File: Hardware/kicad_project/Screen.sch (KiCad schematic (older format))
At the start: 9 parts

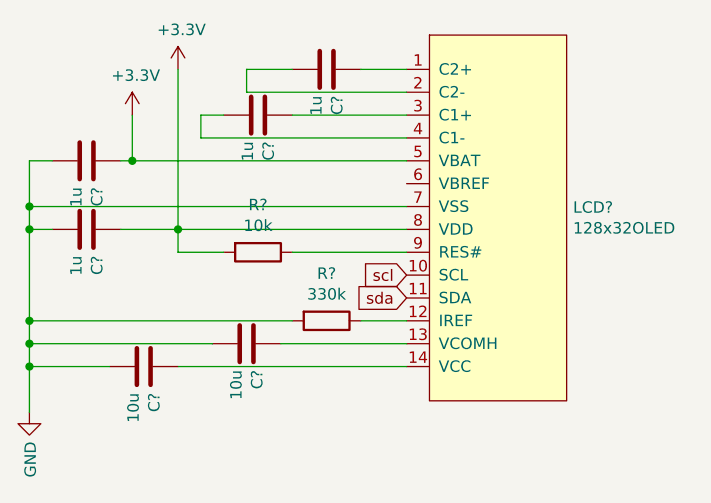
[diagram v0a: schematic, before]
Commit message: update project with corrected schematic / pcb
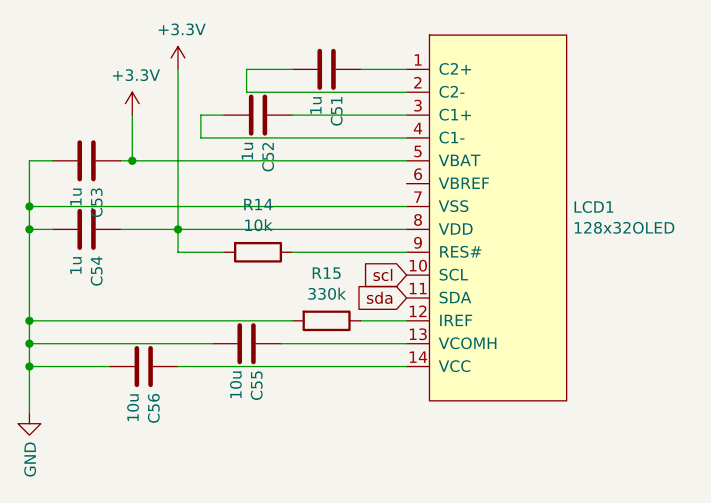
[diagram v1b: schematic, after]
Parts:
- C51, C52, C53, C54: renamed from C?; footprint RandomJunk:C_0603_nosilk -> Capacitors_SMD:C_0402_NoSilk; LCSC c19702 -> C52923
- C55, C56: renamed from C?; footprint RandomJunk:C_0603_nosilk -> Capacitors_SMD:C_0402_NoSilk; LCSC c19702 -> C15525
- LCD1: renamed from LCD?; footprint (none) -> RandomJunk:oled_ssd1306_14pin_91
- R14: renamed from R?; footprint (none) -> Resistors_SMD:R_0402_NoSilk; LCSC (none) -> C25744
- R15: renamed from R?; footprint (none) -> Resistors_SMD:R_0402_NoSilk; LCSC (none) -> C25778
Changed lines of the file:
@@
 sda
 $Comp
-L customLibrary:128x32OLED LCD?
+L customLibrary:128x32OLED LCD1
 U 1 1 6364F37E
 P 6500 3750
-F 0 "LCD?" H 6828 3796 50  0000 L CNN
+F 0 "LCD1" H 6828 3796 50  0000 L CNN
 F 1 "128x32OLED" H 6828 3705 50  0000 L CNN
-F 2 "" H 6550 3800 50  0001 C CNN
+F 2 "RandomJunk:oled_ssd1306_14pin_91" H 6550 3800 50  0001 C CNN
 F 3 "" H 6550 3800 50  0001 C CNN
 	1    6500 3750
@@
 $EndComp
 $Comp
-L Device:C C?
+L Device:C C51
 U 1 1 6364F385
 P 5750 3100
-F 0 "C?" H 5865 3146 50  0000 L CNN
+F 0 "C51" H 5865 3146 50  0000 L CNN
 F 1 "1u" H 5865 3055 50  0000 L CNN
-F 2 "RandomJunk:C_0603_nosilk" H 5788 2950 50  0001 C CNN
-F 3 "~" H 5750 3100 50  0001 C CNN
-F 4 "c19702" H 5750 3100 50  0001 C CNN "LCSC"
+F 2 "Capacitors_SMD:C_0402_NoSilk" H 5788 2950 50  0001 C CNN
+F 3 "" H 5750 3100 50  0001 C CNN
+F 4 "C52923" H 5750 3100 50  0001 C CNN "LCSC"
 	1    5750 3100
 	0    1    1    0
 $EndComp
 $Comp
-L Device:C C?
+L Device:C C52
 U 1 1 6364F38C
 P 5450 3300
-F 0 "C?" H 5565 3346 50  0000 L CNN
+F 0 "C52" H 5565 3346 50  0000 L CNN
 F 1 "1u" H 5565 3255 50  0000 L CNN
-F 2 "RandomJunk:C_0603_nosilk" H 5488 3150 50  0001 C CNN
+F 2 "Capacitors_SMD:C_0402_NoSilk" H 5488 3150 50  0001 C CNN
 F 3 "~" H 5450 3300 50  0001 C CNN
-F 4 "c19702" H 5450 3300 50  0001 C CNN "LCSC"
+F 4 "C52923" H 5450 3300 50  0001 C CNN "LCSC"
 	1    5450 3300
 	0    1    1    0
@@
 	5200 3400 6100 3400
 $Comp
-L Device:C C?
+L Device:C C53
 U 1 1 6364F39B
 P 4700 3500
-F 0 "C?" H 4815 3546 50  0000 L CNN
+F 0 "C53" H 4815 3546 50  0000 L CNN
 F 1 "1u" H 4815 3455 50  0000 L CNN
-F 2 "RandomJunk:C_0603_nosilk" H 4738 3350 50  0001 C CNN
+F 2 "Capacitors_SMD:C_0402_NoSilk" H 4738 3350 50  0001 C CNN
 F 3 "~" H 4700 3500 50  0001 C CNN
-F 4 "c19702" H 4700 3500 50  0001 C CNN "LCSC"
+F 4 "C52923" H 4700 3500 50  0001 C CNN "LCSC"
 	1    4700 3500
 	0    1    1    0
 $EndComp
 $Comp
-L Device:C C?
+L Device:C C54
 U 1 1 6364F3A2
 P 4700 3800
-F 0 "C?" H 4815 3846 50  0000 L CNN
+F 0 "C54" H 4815 3846 50  0000 L CNN
 F 1 "1u" H 4815 3755 50  0000 L CNN
-F 2 "RandomJunk:C_0603_nosilk" H 4738 3650 50  0001 C CNN
+F 2 "Capacitors_SMD:C_0402_NoSilk" H 4738 3650 50  0001 C CNN
 F 3 "~" H 4700 3800 50  0001 C CNN
-F 4 "c19702" H 4700 3800 50  0001 C CNN "LCSC"
+F 4 "C52923" H 4700 3800 50  0001 C CNN "LCSC"
 	1    4700 3800
 	0    1    1    0
 $EndComp
 $Comp
-L power:+3.3V #PWR?
+L power:+3.3V #PWR039
 U 1 1 6364F3A8
 P 4900 3300
-F 0 "#PWR?" H 4900 3150 50  0001 C CNN
+F 0 "#PWR039" H 4900 3150 50  0001 C CNN
 F 1 "+3.3V" H 4915 3473 50  0000 C CNN
 F 2 "" H 4900 3300 50  0001 C CNN
@@
 $EndComp
 $Comp
-L power:+3.3V #PWR?
+L power:+3.3V #PWR038
 U 1 1 6364F3AE
 P 5100 3100
-F 0 "#PWR?" H 5100 2950 50  0001 C CNN
+F 0 "#PWR038" H 5100 2950 50  0001 C CNN
 F 1 "+3.3V" H 5115 3273 50  0000 C CNN
 F 2 "" H 5100 3100 50  0001 C CNN
@@
 	5100 3800 6100 3800
 $Comp
-L power:GND #PWR?
+L power:GND #PWR040
 U 1 1 6364F3BB
 P 4450 4600
-F 0 "#PWR?" H 4450 4350 50  0001 C CNN
+F 0 "#PWR040" H 4450 4350 50  0001 C CNN
 F 1 "GND" V 4455 4472 50  0000 R CNN
 F 2 "" H 4450 4600 50  0001 C CNN
@@
 $EndComp
 $Comp
-L Device:C C?
+L Device:C C56
 U 1 1 6364F3C2
 P 4950 4400
-F 0 "C?" H 5065 4446 50  0000 L CNN
+F 0 "C56" H 5065 4446 50  0000 L CNN
 F 1 "10u" H 5065 4355 50  0000 L CNN
-F 2 "RandomJunk:C_0603_nosilk" H 4988 4250 50  0001 C CNN
+F 2 "Capacitors_SMD:C_0402_NoSilk" H 4988 4250 50  0001 C CNN
 F 3 "~" H 4950 4400 50  0001 C CNN
-F 4 "c19702" H 4950 4400 50  0001 C CNN "LCSC"
+F 4 "C15525" H 4950 4400 50  0001 C CNN "LCSC"
 	1    4950 4400
 	0    1    1    0
 $EndComp
 $Comp
-L Device:C C?
+L Device:C C55
 U 1 1 6364F3C9
 P 5400 4300
-F 0 "C?" H 5515 4346 50  0000 L CNN
+F 0 "C55" H 5515 4346 50  0000 L CNN
 F 1 "10u" H 5515 4255 50  0000 L CNN
-F 2 "RandomJunk:C_0603_nosilk" H 5438 4150 50  0001 C CNN
+F 2 "Capacitors_SMD:C_0402_NoSilk" H 5438 4150 50  0001 C CNN
 F 3 "~" H 5400 4300 50  0001 C CNN
-F 4 "c19702" H 5400 4300 50  0001 C CNN "LCSC"
+F 4 "C15525" H 5400 4300 50  0001 C CNN "LCSC"
 	1    5400 4300
 	0    1    1    0
 $EndComp
 $Comp
-L Device:R R?
+L Device:R R15
 U 1 1 6364F3CF
 P 5750 4200
-F 0 "R?" V 5543 4200 50  0000 C CNN
+F 0 "R15" V 5543 4200 50  0000 C CNN
 F 1 "330k" V 5634 4200 50  0000 C CNN
-F 2 "" V 5680 4200 50  0001 C CNN
+F 2 "Resistors_SMD:R_0402_NoSilk" V 5680 4200 50  0001 C CNN
 F 3 "~" H 5750 4200 50  0001 C CNN
+F 4 "C25778" H 5750 4200 50  0001 C CNN "LCSC"
 	1    5750 4200
 	0    1    1    0
@@
 	4450 3700 4450 3800
 $Comp
-L Device:R R?
+L Device:R R14
 U 1 1 6364F3E9
 P 5450 3900
-F 0 "R?" V 5243 3900 50  0000 C CNN
+F 0 "R14" V 5243 3900 50  0000 C CNN
 F 1 "10k" V 5334 3900 50  0000 C CNN
-F 2 "" V 5380 3900 50  0001 C CNN
+F 2 "Resistors_SMD:R_0402_NoSilk" V 5380 3900 50  0001 C CNN
 F 3 "~" H 5450 3900 50  0001 C CNN
+F 4 "C25744" H 5450 3900 50  0001 C CNN "LCSC"
 	1    5450 3900
 	0    1    1    0
